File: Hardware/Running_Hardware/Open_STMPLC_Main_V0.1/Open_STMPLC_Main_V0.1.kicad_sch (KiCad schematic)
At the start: 8 parts

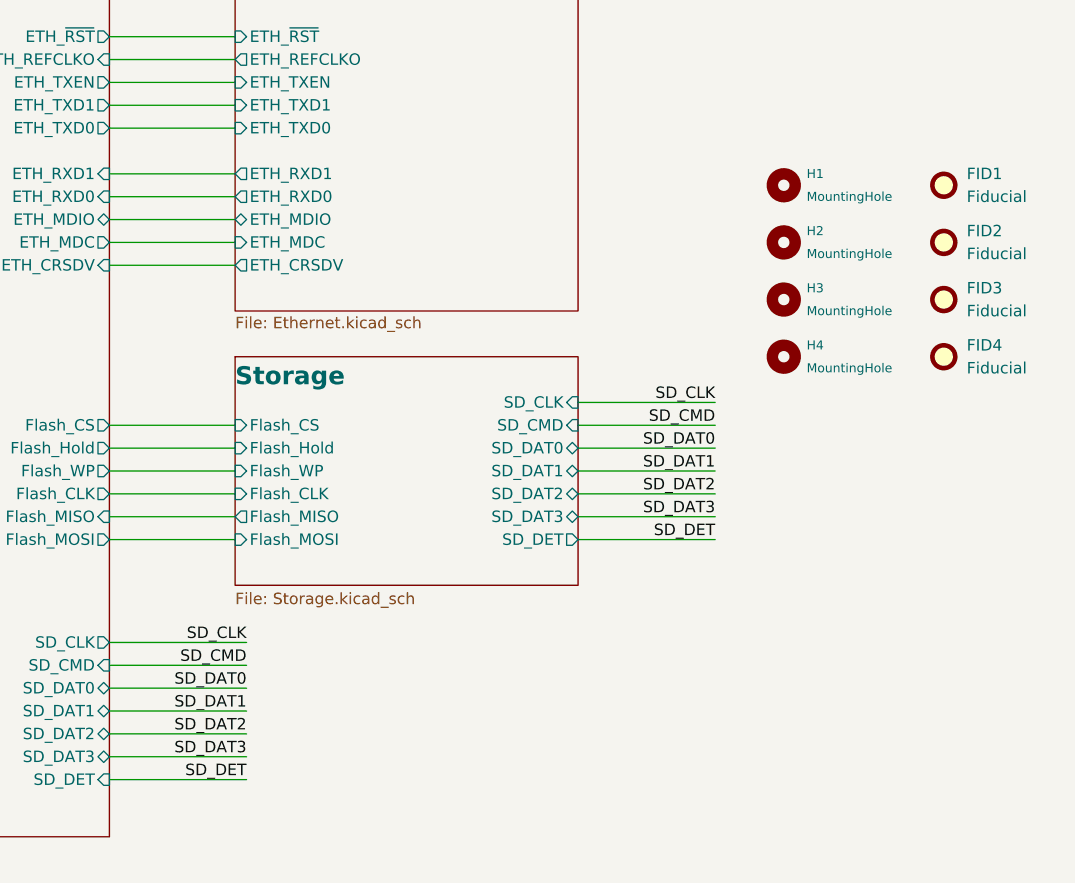
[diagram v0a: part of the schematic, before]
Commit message: Silkscreen and DRC
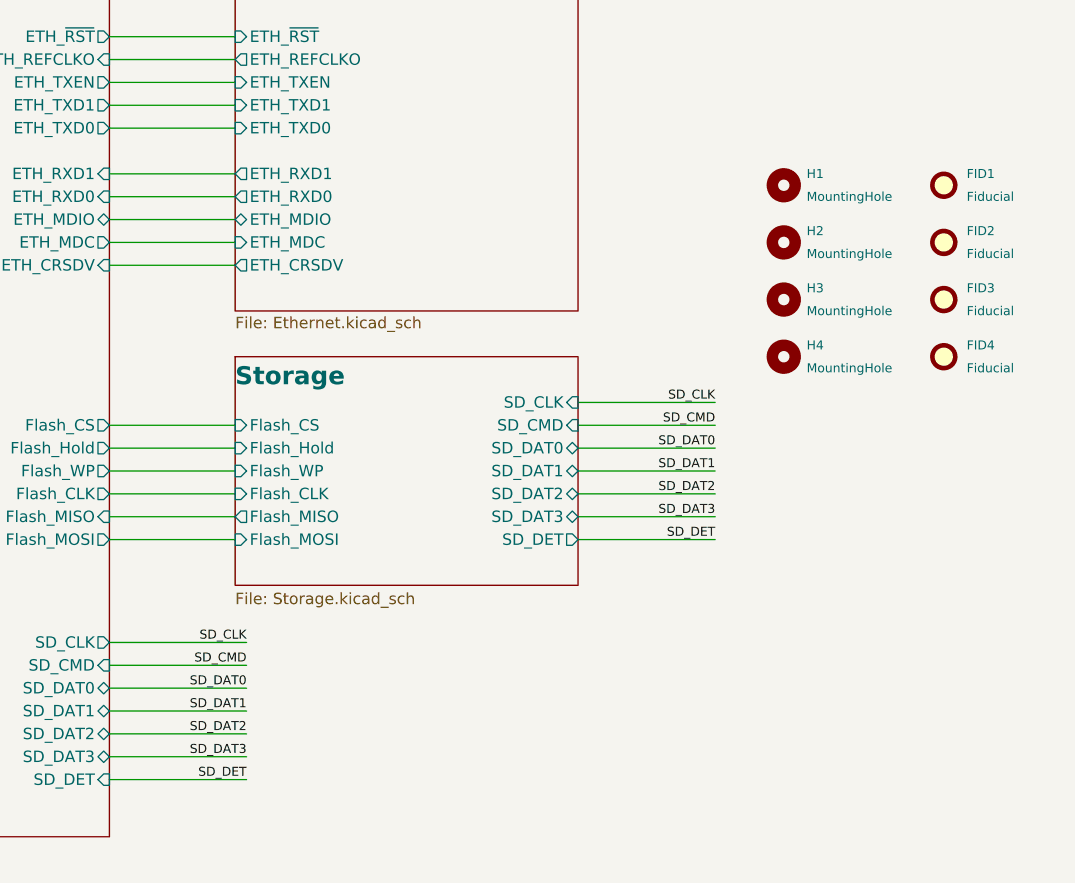
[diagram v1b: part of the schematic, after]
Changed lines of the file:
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@@
 	(title_block
 		(title "Open_STMPLC_Main")
-		(date "2026-05-23")
+		(date "2026-05-24")
 		(rev "0.1")
 	)
@@
 		(effects
 			(font
-				(size 1.27 1.27)
+				(size 1 1)
 			)
 			(justify right bottom)
@@
 		(effects
 			(font
-				(size 1.27 1.27)
+				(size 1 1)
 			)
 			(justify right bottom)
@@
 		(effects
 			(font
-				(size 1.27 1.27)
+				(size 1 1)
 			)
 			(justify right bottom)
@@
 		(effects
 			(font
-				(size 1.27 1.27)
+				(size 1 1)
 			)
 			(justify right bottom)
@@
 		(effects
 			(font
-				(size 1.27 1.27)
+				(size 1 1)
 			)
 			(justify right bottom)
@@
 		(effects
 			(font
-				(size 1.27 1.27)
+				(size 1 1)
 			)
 			(justify right bottom)
@@
 		(effects
 			(font
-				(size 1.27 1.27)
+				(size 1 1)
 			)
 			(justify right bottom)
@@
 		(effects
 			(font
-				(size 1.27 1.27)
+				(size 1 1)
 			)
 			(justify right bottom)
@@
 		(effects
 			(font
-				(size 1.27 1.27)
+				(size 1 1)
 			)
 			(justify right bottom)
@@
 		(effects
 			(font
-				(size 1.27 1.27)
+				(size 1 1)
 			)
 			(justify right bottom)
@@
 		(effects
 			(font
-				(size 1.27 1.27)
+				(size 1 1)
 			)
 			(justify right bottom)
@@
 		(effects
 			(font
-				(size 1.27 1.27)
+				(size 1 1)
 			)
 			(justify right bottom)
@@
 		(effects
 			(font
-				(size 1.27 1.27)
+				(size 1 1)
 			)
 			(justify right bottom)
@@
 		(effects
 			(font
-				(size 1.27 1.27)
+				(size 1 1)
 			)
 			(justify right bottom)
@@
 			(effects
 				(font
-					(size 1.27 1.27)
+					(size 1 1)
 				)
 				(justify left)
@@
 			(effects
 				(font
-					(size 1.27 1.27)
+					(size 1 1)
 				)
 				(justify left)
@@
 			(effects
 				(font
-					(size 1.27 1.27)
+					(size 1 1)
 				)
 				(justify left)
@@
 			(effects
 				(font
-					(size 1.27 1.27)
+					(size 1 1)
 				)
 				(justify left)
@@
 			(effects
 				(font
-					(size 1.27 1.27)
+					(size 1 1)
 				)
 				(justify left)
@@
 			(effects
 				(font
-					(size 1.27 1.27)
+					(size 1 1)
 				)
 				(justify left)
@@
 			(effects
 				(font
-					(size 1.27 1.27)
+					(size 1 1)
 				)
 				(justify left)
@@
 			(effects
 				(font
-					(size 1.27 1.27)
+					(size 1 1)
 				)
 				(justify left)
